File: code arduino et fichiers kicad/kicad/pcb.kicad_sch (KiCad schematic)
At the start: 37 parts, among them J1 Screw_Terminal_01x04, J2 Screw_Terminal_01x04, J3 Screw_Terminal_01x02, U1 LMC6482, U2 LMC6482, U3 LMC6482

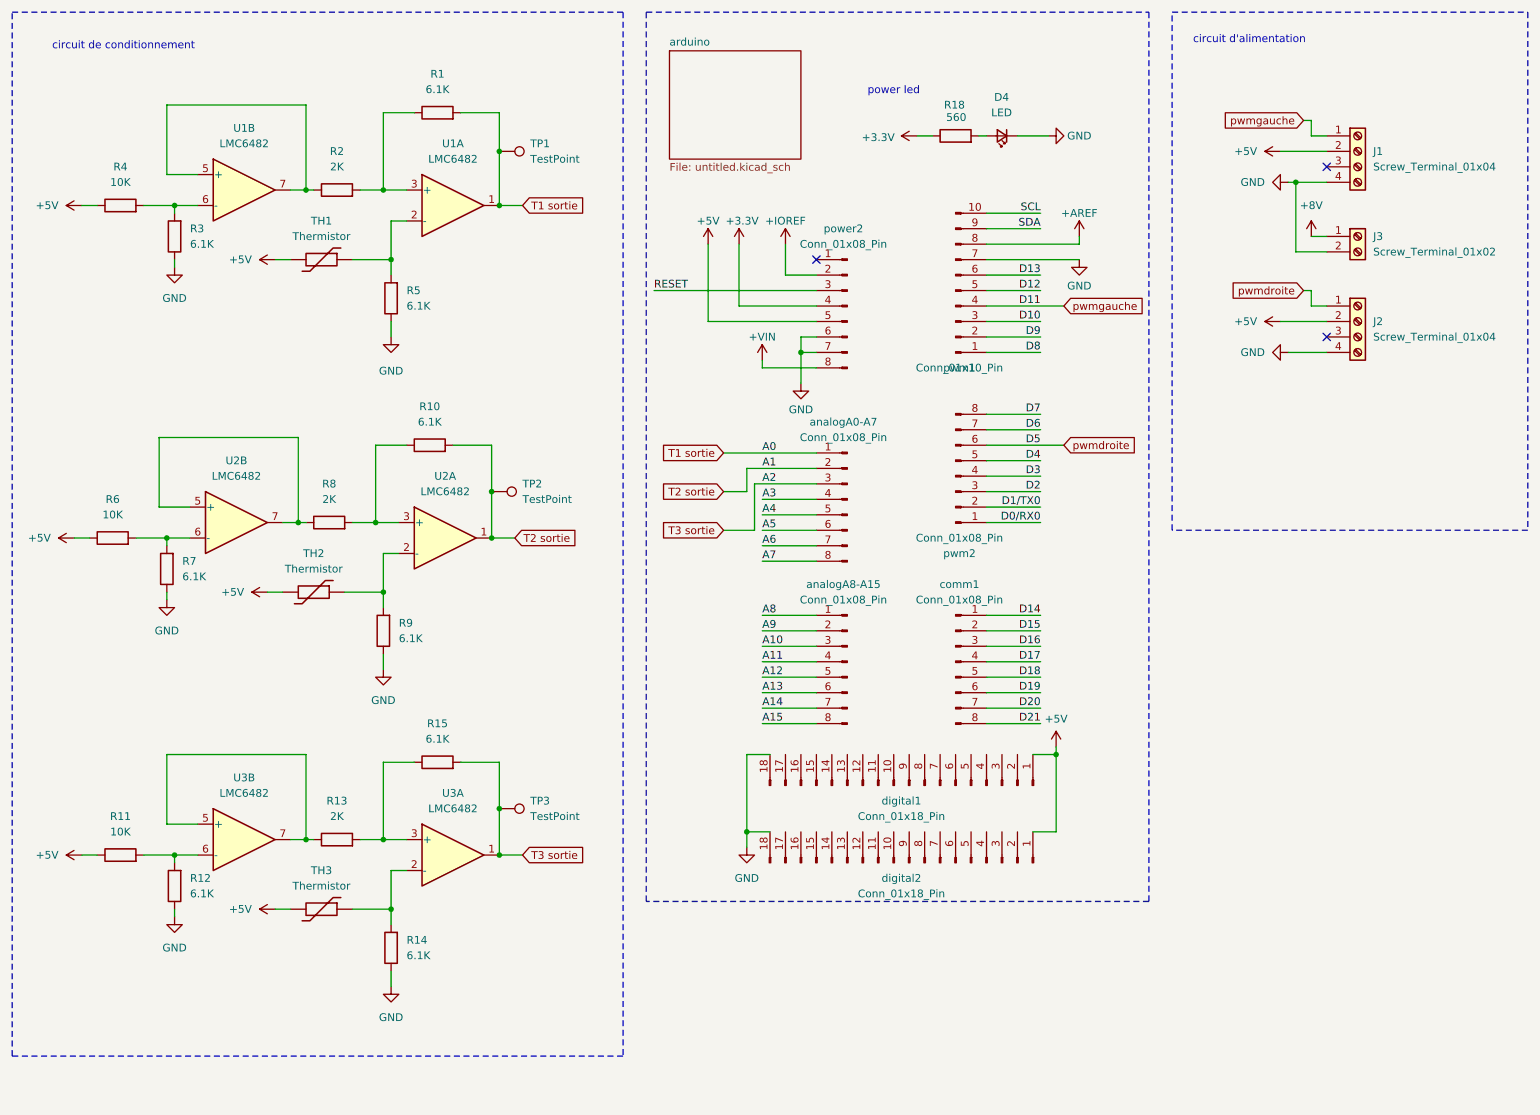
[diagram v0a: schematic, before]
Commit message: version tht pour pas trop haïr notre vie plus tard
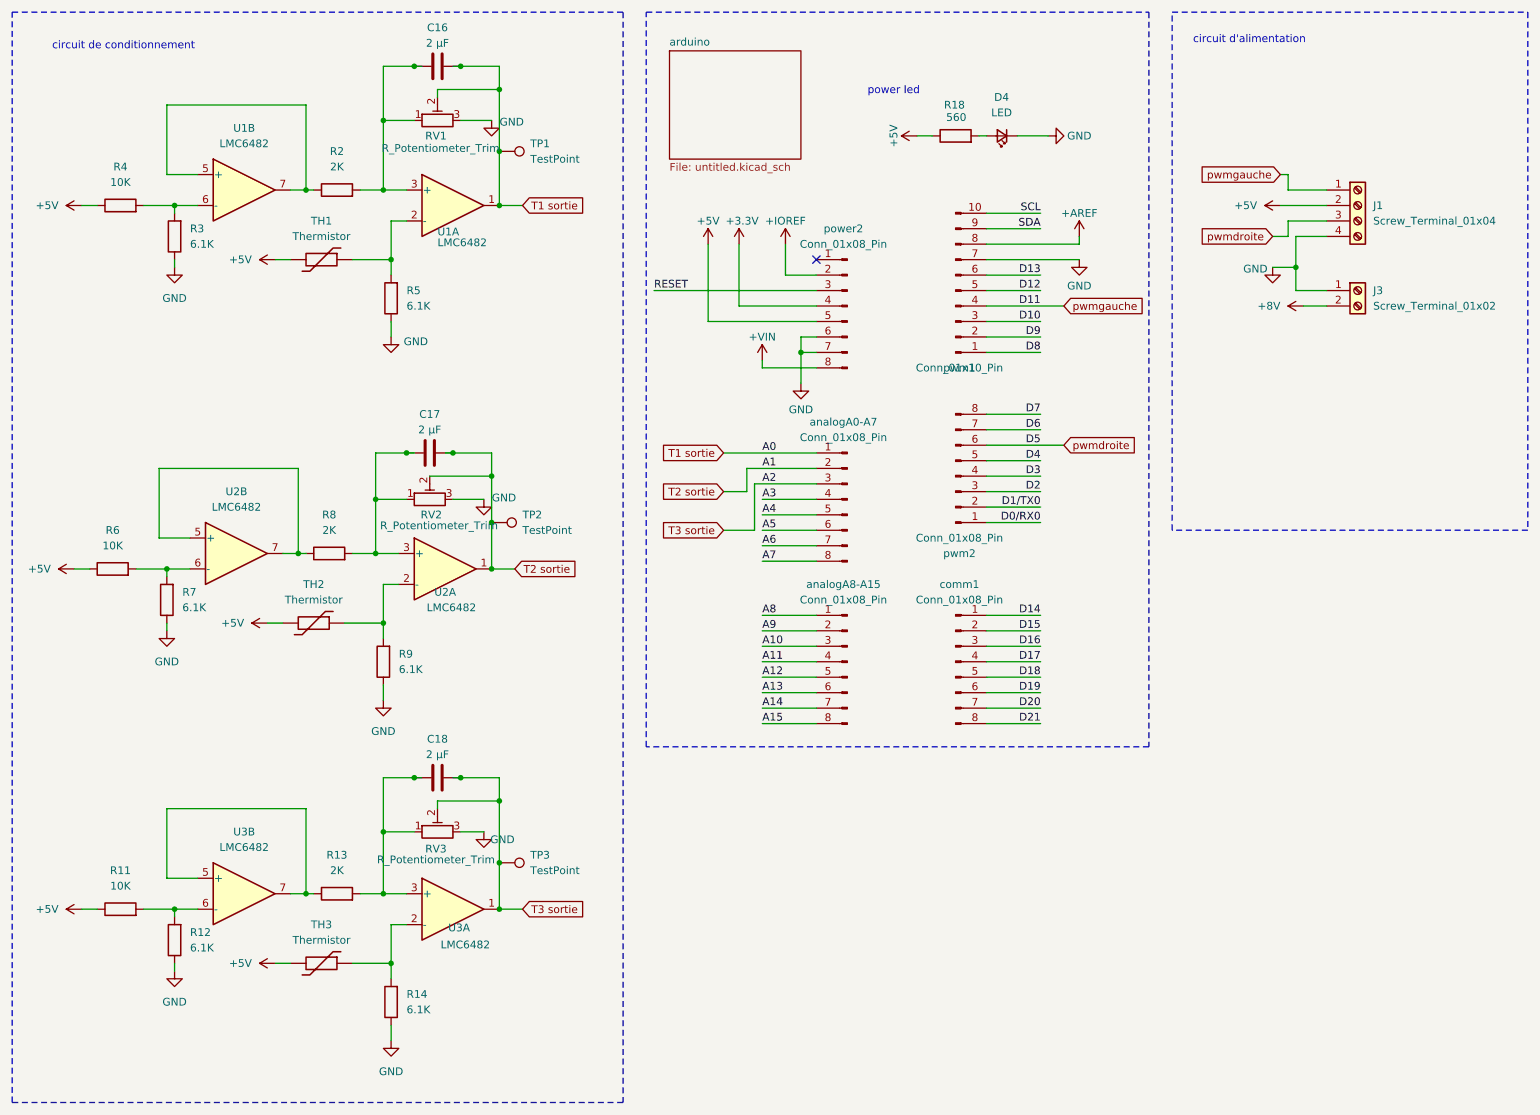
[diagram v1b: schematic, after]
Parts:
- removed J2: Screw_Terminal_01x04, Connector_JST:JST_XH_B4B-XH-A_1x04_P2.50mm_Vertical, symbol Connector:Screw_Terminal_01x04
- removed R1, R10, R15: 6.1K, Resistor_SMD:R_0805_2012Metric_Pad1.20x1.40mm_HandSolder, symbol Device:R
- removed digital1, digital2: Conn_01x18_Pin, Connector_PinHeader_2.54mm:PinHeader_1x18_P2.54mm_Vertical, symbol Connector:Conn_01x18_Pin
- added C16, C17, C18: 2 μF, Capacitor_THT:CP_Radial_D5.0mm_P2.50mm, symbol Device:C
- added RV1, RV2, RV3: R_Potentiometer_Trim, Library:trimpot, symbol Device:R_Potentiometer_Trim
- D4: footprint PCM_SparkFun-LED:LED_0603_1608Metric -> LED_THT:LED_D5.0mm
- R11, R12, R13, R14, R18, R2, R3, R4, R5, R6, R7, R8, R9: footprint Resistor_SMD:R_0805_2012Metric_Pad1.20x1.40mm_HandSolder -> Resistor_THT:R_Axial_DIN0207_L6.3mm_D2.5mm_P7.62mm_Horizontal
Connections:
- net +3.3V: no longer R18.1
- net +5V: now also R18.1
- net +8V: now also J3.2 (Pin_2); no longer J3.1 (Pin_1)
- net GND: now also J3.1 (Pin_1), RV1.3, RV2.3, RV3.3; no longer J3.2 (Pin_2)
- net T1 sortie: now also C16.2, RV1.2
- net T2 sortie: now also C17.2, RV2.2
- net T3 sortie: now also C18.2, RV3.2
- net pwmdroite: now also J1.3 (Pin_3)
- net at R2.2, U1.3 (+): now also C16.1, RV1.1
- net at R8.2, U2.3 (+): now also C17.1, RV2.1
- net at R13.2, U3.3 (+): now also C18.1, RV3.1
- no-connect marks 3 -> 1
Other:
- moved on the sheet: J1, J3, R11, R12, R13, R14, R6, R7, R8, R9, TH2, TH3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
